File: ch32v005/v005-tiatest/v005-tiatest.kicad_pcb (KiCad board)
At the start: 2 copper layers, 19 x 22 mm, 9 parts, among them J1 HDR

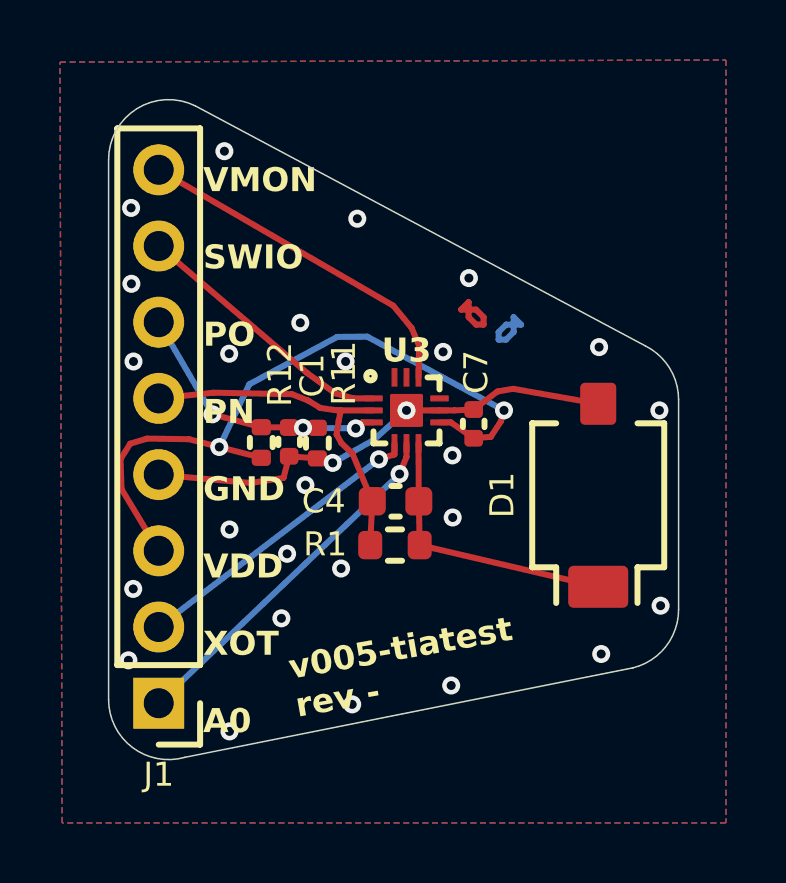
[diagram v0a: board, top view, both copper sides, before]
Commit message: Update tiatest with functional rev
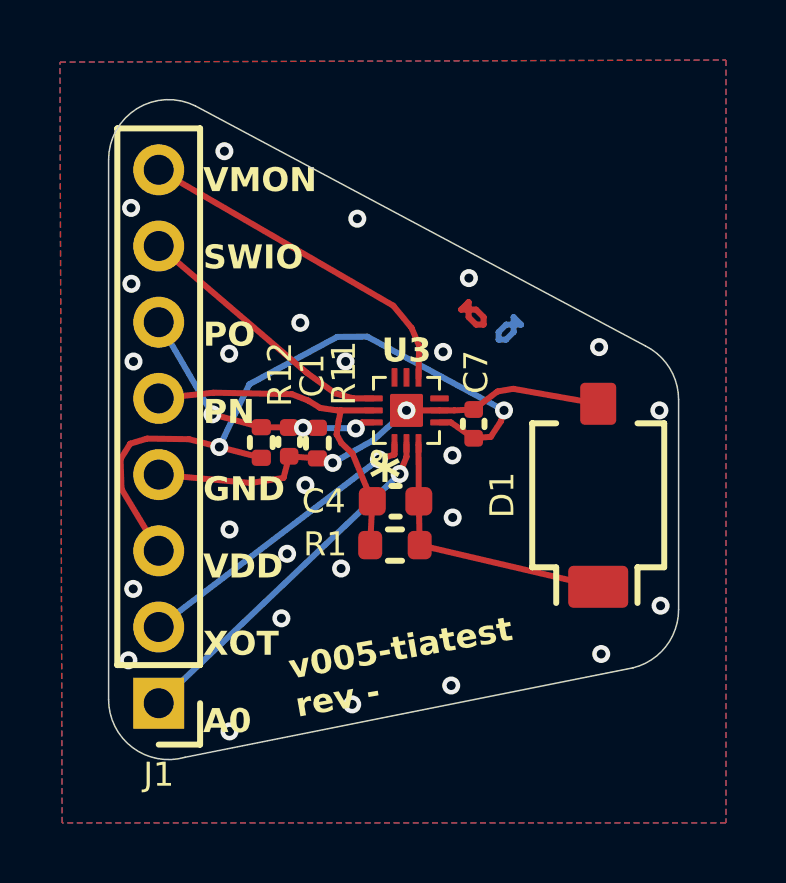
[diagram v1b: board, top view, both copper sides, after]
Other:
- board text added: "*"
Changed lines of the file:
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@@
 		(attr smd)
+		(fp_line
+			(start -1.1 -1.1)
+			(end -0.7 -1.1)
+			(stroke
+				(width 0.1)
+				(type default)
+			)
+			(layer "F.SilkS")
+		)
+		(fp_line
+			(start -1.1 -0.7)
+			(end -1.1 -1.1)
+			(stroke
+				(width 0.1)
+				(type default)
+			)
+			(layer "F.SilkS")
+		)
 		(fp_line
 			(start -1.1 1.1)
 			(end -1.1 0.7)
 			(stroke
-				(width 0.2)
+				(width 0.1)
 				(type default)
 			)
@@
 			(end -1.1 1.1)
 			(stroke
-				(width 0.2)
+				(width 0.1)
 				(type default)
 			)
@@
 			(end 1.1 -1.1)
 			(stroke
-				(width 0.2)
+				(width 0.1)
 				(type default)
 			)
@@
 			(end 1.1 -0.7)
 			(stroke
-				(width 0.2)
+				(width 0.1)
 				(type default)
 			)
@@
 			(end 1.1 1.1)
 			(stroke
-				(width 0.2)
+				(width 0.1)
 				(type default)
 			)
@@
 			(end 0.7 1.1)
 			(stroke
-				(width 0.2)
+				(width 0.1)
 				(type default)
 			)
@@
 		)
 		(fp_circle
-			(center -1.2 -1.141421)
-			(end -1.1 -1.041421)
-			(stroke
-				(width 0.2)
+			(center -1 1.5)
+			(end -0.9 1.6)
+			(stroke
+				(width 0.1)
 				(type default)
 			)
@@
 		)
 	)
+	(gr_text "*"
+		(at 121.75 88.5 0)
+		(layer "F.SilkS")
+		(effects
+			(font
+				(size 1.5 1.5)
+				(thickness 0.3)
+				(bold yes)
+			)
+			(justify left bottom mirror)
+		)
+	)
